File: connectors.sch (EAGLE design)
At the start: 19 parts, among them CON1 CON-4P-JST_GH-RA, CON2 CON-4P-JST_GH-RA, CON20 PINHEAD_1X03-2.54-RA, CON4 PINHEAD_1X02-2, CON5 PINHEAD_1X02-2, CON6 PINHEAD_1X07-2, IC1 TJA1051, IC2 TPD3S014DBVR-SOT23-6

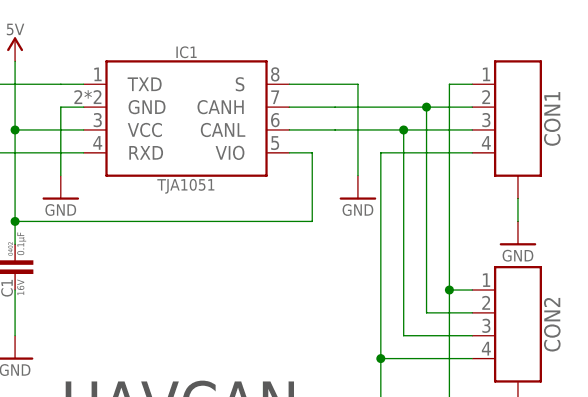
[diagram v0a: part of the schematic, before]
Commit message: Library update
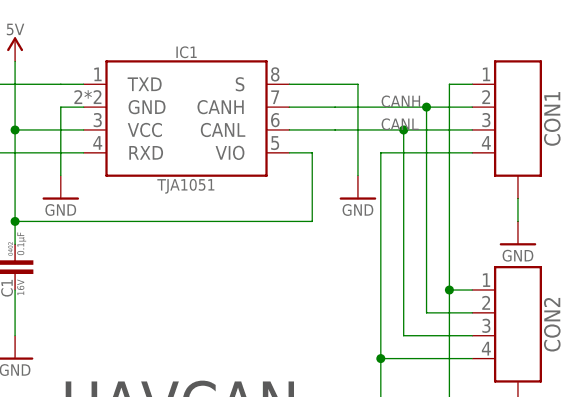
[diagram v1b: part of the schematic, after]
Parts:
- CON1, CON2: value CON-4P-JST_GH-RA -> CON-4P-TABS-JST_GH-RA; device Connectors:CON-4P-JST_GH-RA -> Connectors:CON-4P-TABS-JST_GH-RA
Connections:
- net N$23 renamed CANH
- net N$35 renamed CANL
